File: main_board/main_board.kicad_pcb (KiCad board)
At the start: 2 copper layers, 145 x 87 mm, 137 parts, among them J1 stepper0, J10 24VDCout5, J11 5VDCout0, J12 5VDCout1, J13 5VDCout2, J14 5VDCout3, J15 5VDCout4, J16 5VDCout5, J17 temp0, J18 temp1, J19 I2C, J2 stepper1, J20 I2C, J21 I2C, J22 I2C, J23 analogIn0, J24 weightSensor, J25 lightSensor, J26 24VDC_in, J27 24VDC to 5VDC step down, J28 24VDC, J29 24VDC, J3 stepper2, J30 24VDC, J31 5VDC, J32 5VDC, J33 5VDC, J34 analogIn1, J35 reflectiveSensor, J36 24VDC, J37 24VDC, J38 24VDC, J39 5VDC, J4 stepper3, J40 5VDC, J41 5VDC, J42 encoder, J5 24VDCout0, J6 24VDCout1, J7 24VDCout2, J8 24VDCout3, J9 24VDCout4, Q1 Q_NMOS_GDS, Q10 BS170, Q11 BS170, Q12 BS170, Q2 Q_NMOS_GDS, Q3 Q_NMOS_GDS, Q4 Q_NMOS_GDS, Q5 Q_NMOS_GDS, Q6 Q_NMOS_GDS, Q7 BS170, Q8 BS170, Q9 BS170, U1 ESP32-DEVKITC-32D, U2 PCA9685PW

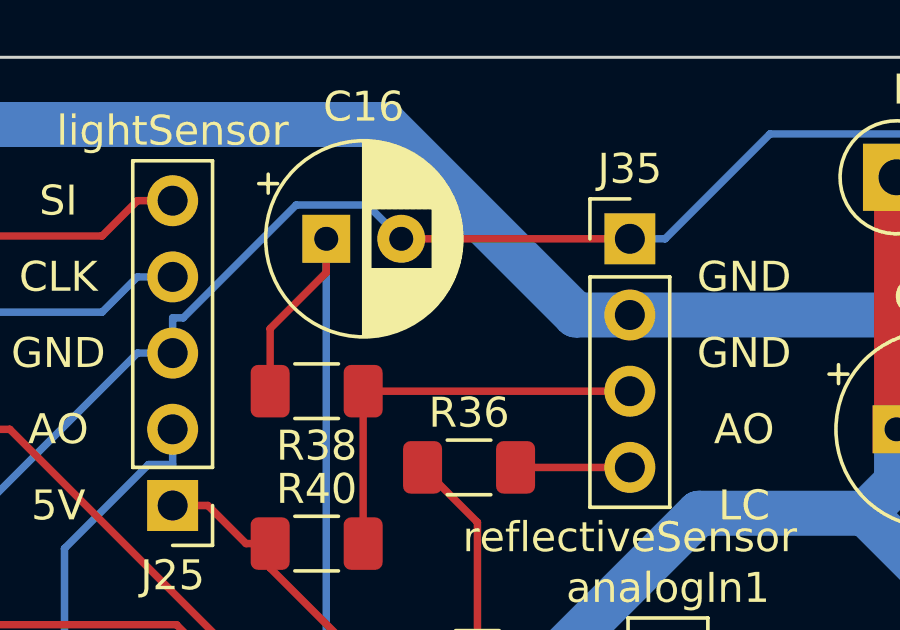
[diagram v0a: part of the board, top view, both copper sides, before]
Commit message: bug fix
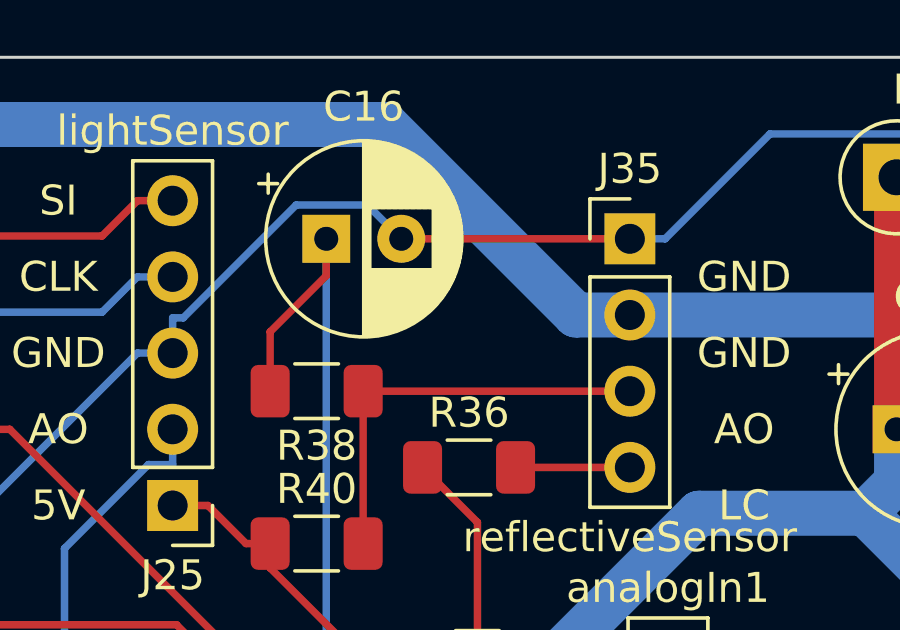
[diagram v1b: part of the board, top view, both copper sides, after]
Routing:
- net reflectiveSensor0: track 0.00 -> 5.85 mm
- net reflectivesensor0: track 43.9 -> 38.1 mm
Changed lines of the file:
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@@
   (segment (start 107.99 19.05) (end 107.99 35.52) (width 0.25) (layer B.Cu) (net 52))
   (segment (start 107.99 35.52) (end 92.71 50.8) (width 0.25) (layer B.Cu) (net 52))
-  (segment (start 107.99 19.05) (end 107.99 20.1753) (width 0.25) (layer F.Cu) (net 52))
-  (segment (start 106.12 24.13) (end 106.12 22.0453) (width 0.25) (layer F.Cu) (net 52))
-  (segment (start 106.12 22.0453) (end 107.99 20.1753) (width 0.25) (layer F.Cu) (net 52))
   (segment (start 163.83 77.47) (end 163.83 78.9153) (width 0.25) (layer F.Cu) (net 53))
   (segment (start 163.9034 82.4766) (end 162.56 83.82) (width 0.25) (layer F.Cu) (net 53))
@@
   (segment (start 118.11 26.67) (end 114.3 26.67) (width 0.25) (layer F.Cu) (net 73))
   (segment (start 109.22 24.13) (end 109.22 29.21) (width 0.25) (layer F.Cu) (net 74))
-  (segment (start 118.11 24.13) (end 109.22 24.13) (width 0.25) (layer F.Cu) (net 74))
+  (segment (start 109.22 24.13) (end 118.11 24.13) (width 0.25) (layer F.Cu) (net 74))
   (segment (start 160.02 83.82) (end 160.02 78.74) (width 0.25) (layer F.Cu) (net 75))
   (segment (start 160.02 78.74) (end 158.75 77.47) (width 0.25) (layer F.Cu) (net 75))
@@
   (segment (start 110.1996 35.8504) (end 110.1996 33.02) (width 0.25) (layer B.Cu) (net 117))
   (via (at 110.1996 33.02) (size 0.8) (layers F.Cu B.Cu) (net 117))
+  (segment (start 107.99 19.05) (end 107.99 20.28) (width 0.25) (layer F.Cu) (net 118))
+  (segment (start 106.12 22.15) (end 106.12 24.13) (width 0.25) (layer F.Cu) (net 118))
+  (segment (start 107.99 20.28) (end 106.12 22.15) (width 0.25) (layer F.Cu) (net 118))
   (segment (start 138.43 53.34) (end 137.2046 54.5654) (width 0.25) (layer F.Cu) (net 119))
   (segment (start 137.2046 54.5654) (end 133.0254 54.5654) (width 0.25) (layer F.Cu) (net 119))
